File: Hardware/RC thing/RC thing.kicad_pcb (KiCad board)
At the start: 2 copper layers, 56.4 x 52.8 mm, 68 parts, among them J1 Conn_01x04, J2 2171790001, SW1 Bat_switch, SW1 TL3342F160QG_TR, SW2 SW_Push, SW3 SW_Push, SW4 SW_Push, SW5 TL3342F160QG_TR, U1 MCP73831-2-OT, U101 NRF24L01_Breakout, U2 RP2040, U3 W25Q128JVS, U401 TPS62170DSG, Y3 Crystal_GND24_Small

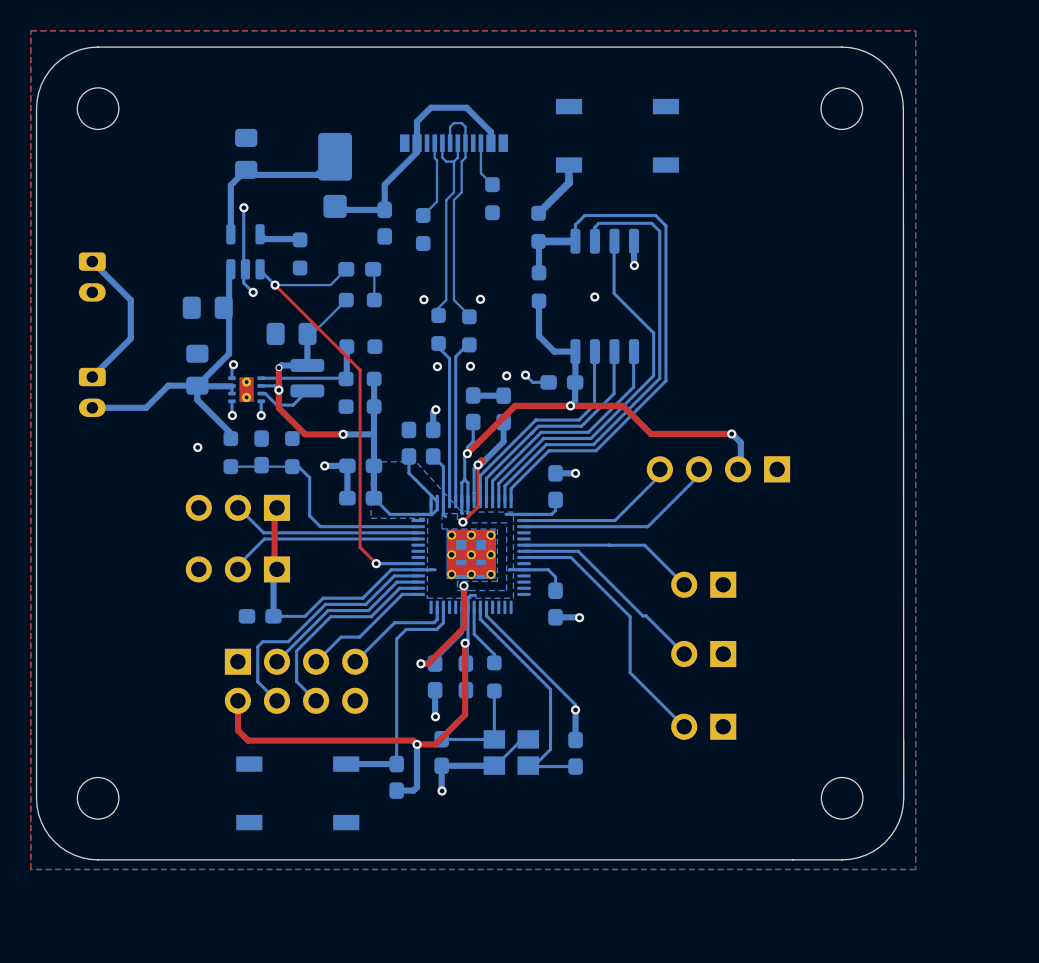
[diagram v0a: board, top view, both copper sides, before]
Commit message: new RC PCB updates
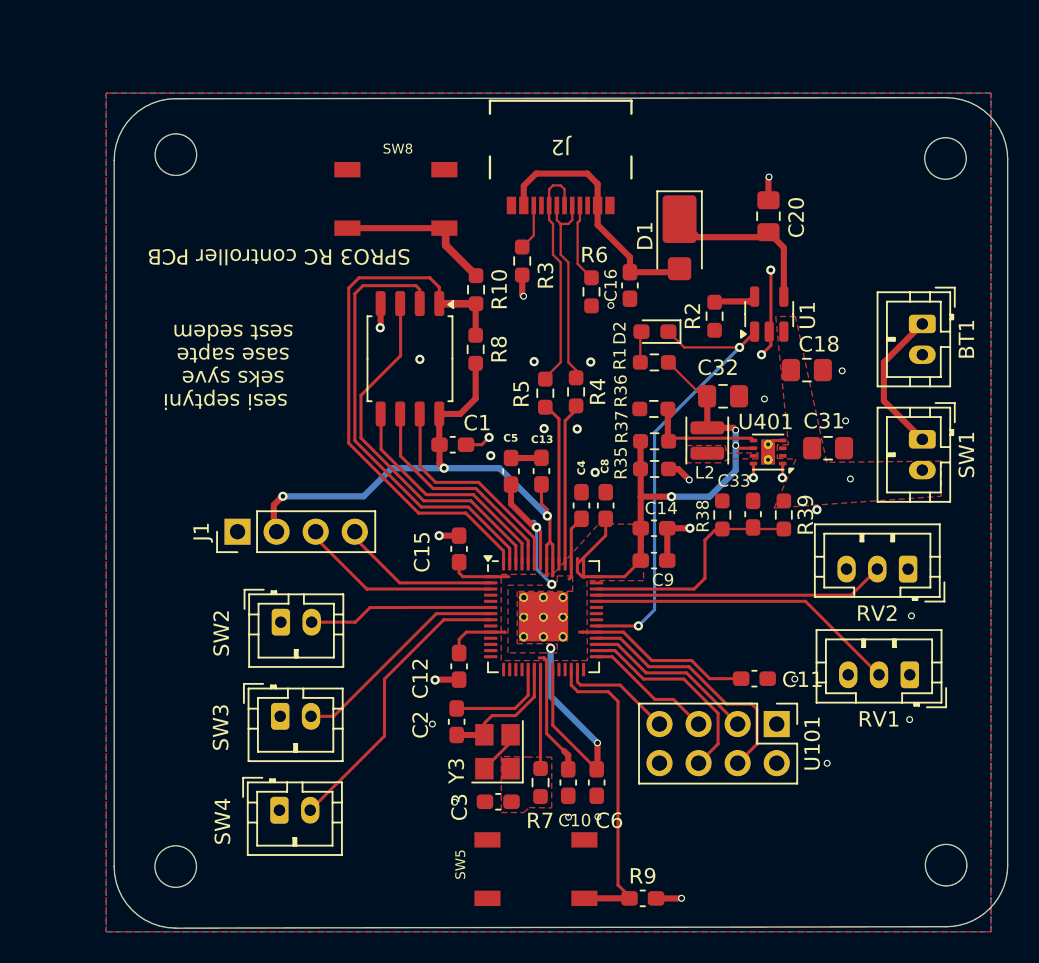
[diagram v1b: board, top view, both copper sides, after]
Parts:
- removed the R1 at (135.3, 88.5)
- removed the SW1 at (128.8, 89.5)
- added R9: 10k, Capacitor_SMD:C_0603_1608Metric_Pad1.08x0.95mm_HandSolder, F.Cu at (151.3, 96.4)
- added SW8: TL3342F160QG_TR, Main_PCB:SW_TL3342F160QG_TR, F.Cu at (135.2, 50.9)
- ? (x9), H1, H2, H3, H4: moved to B.Cu
- BT1, C1, C10, C11, C12, C13, C14, C15, C16, C18, C2, C20, C3, C4, C5, C6, C8, C9, D1, D2, J1, J2, R1, R10, R2, R3, R4, R5, R6, R7, R8, SW1, SW5, U1, U101, U2, U3, U401, Y3: moved to F.Cu
- C31: renamed from C401; moved to F.Cu
- C32: renamed from C404; moved to F.Cu
- C33: renamed from C409; moved to F.Cu
- L2: renamed from L402; moved to F.Cu
- R35: renamed from R403; moved to F.Cu
- R36: renamed from R405; moved to F.Cu
- R37: renamed from R404; moved to F.Cu
- R38: renamed from R411; moved to F.Cu
- R39: renamed from R410; moved to F.Cu
- RV1, RV2: footprint Connector_PinHeader_2.54mm:PinHeader_1x03_P2.54mm_Vertical -> Connector_JST:JST_PH_B3B-PH-K_1x03_P2.00mm_Vertical; moved to F.Cu
- SW2, SW3, SW4: footprint Connector_PinHeader_2.54mm:PinHeader_1x02_P2.54mm_Vertical -> Connector_JST:JST_PH_B2B-PH-K_1x02_P2.00mm_Vertical; moved to F.Cu
- moved H4 55.3 mm to (171.0, 94.2), turned to 180 degrees
- moved H1 55.2 mm to (170.9, 48.3), turned to 180 degrees
- moved BT1 54.1 mm to (169.4, 59.0)
- moved SW1 54.1 mm to (169.4, 66.5)
- moved SW5 47.9 mm to (144.3, 94.5), turned to 0 degrees
- moved H3 43.5 mm to (120.9, 94.3), turned to 180 degrees
- moved H2 43.4 mm to (120.9, 48.0), turned to 180 degrees
- moved RV1 41.7 mm to (168.6, 81.8), turned to 180 degrees
- moved C31 41.3 mm to (163.3, 67.1), turned to 0 degrees
- moved RV2 41.2 mm to (168.5, 75.0), turned to 180 degrees
- moved C18 39.1 mm to (161.9, 62.0), turned to 0 degrees
- moved R39 36.2 mm to (160.4, 71.5)
- moved J1 35.3 mm to (124.9, 72.5)
- moved U101 35.2 mm to (160.0, 85.0)
- moved U1 34.3 mm to (159.5, 58.4)
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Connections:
- SW5 pad 2: /RP2040/~{USB_BOOT} -> /RP2040/RUN
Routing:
- net +3V3: track 133.8 -> 106.4 mm, vias 8 -> 9
- net VBAT: track 22.9 -> 0.00 mm, vias 0 -> 1
- net /RP2040/RUN: track 0.00 -> 20.6 mm
- net Net-(U2-RUN): track 15.9 -> 0.00 mm
- net /RP2040/XIN: track 16.1 -> 8.28 mm
- net /AnaStk_1: track 12.7 -> 20.3 mm
- net Net-(C3-Pad1): track 6.58 -> 0.00 mm
- net /AnaStk_2: track 12.6 -> 19.0 mm
- net /RP2040/~{USB_BOOT}: track 3.96 -> 10.3 mm
- net +1V1: track 26.4 -> 31.4 mm
- net Net-(U401-SW): track 3.70 -> 0.00 mm
- net /RP2040/XOUT: track 4.16 -> 6.43 mm
- net /Button3: track 17.1 -> 19.0 mm
- net +3.3V: track 0.00 -> 1.66 mm, vias 0 -> 1
- net /Button2: track 13.2 -> 14.4 mm
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- added copper zone on F.Cu, net +1V1
- added copper zone on F.Cu, net +3V3
- added copper zone on In2.Cu, net +3V3
- added copper zone on In1.Cu, net GND
- added copper zone on F.Cu, net Net-(C3-Pad1)
- added copper zone on F.Cu, net Net-(U401-SW)
- added copper zone on F.Cu, net VBAT
- removed copper zone on B.Cu, net +1V1
- removed copper zone on B.Cu, net +3V3
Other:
- board size 56.4 x 52.8 mm -> 58.1 x 54 mm
- copper layers 2 -> 4
- board text removed: "->"
- board text removed: "IN ORDER"
- board text removed: "x2"
